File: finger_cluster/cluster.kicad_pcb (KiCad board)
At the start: 2 copper layers, 43.1 x 61 mm, 16 parts, among them J1 Conn_01x06_MountingPin, Q1 BSS84, SW1 SW_SPST, U1 TMAG5263

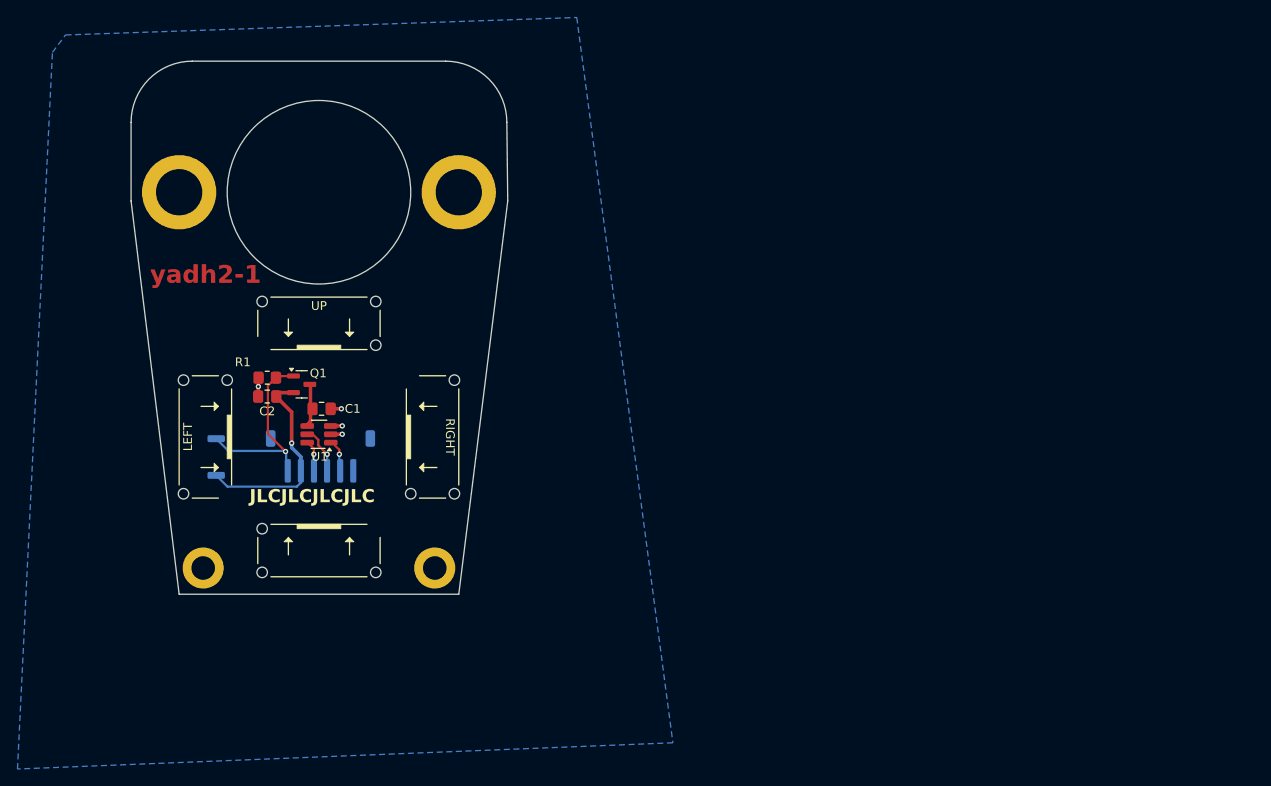
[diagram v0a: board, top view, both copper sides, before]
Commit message: cluster aluminium basic
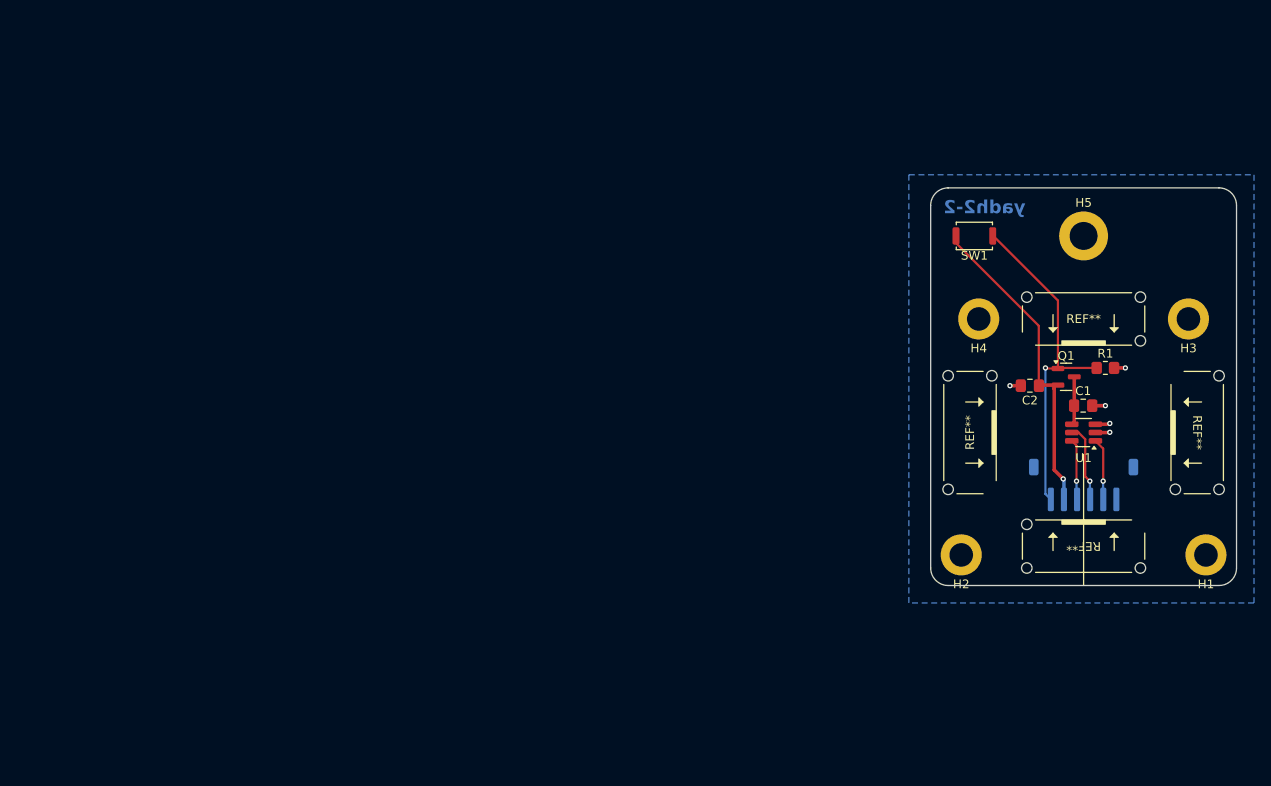
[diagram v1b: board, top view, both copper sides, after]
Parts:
- removed DOWN, LEFT, RIGHT, UP: key, cluster:key
- added H5: MountingHole_Pad, MountingHole:MountingHole_3.2mm_M3_DIN965_Pad, F.Cu at (187.5, 55.0)
- added REF**: key, cluster:key, F.Cu at (172.5, 77.5)
- added REF**: key, cluster:key, F.Cu at (187.5, 92.5)
- added REF**: key, cluster:key, F.Cu at (202.5, 77.5)
- added REF**: key, cluster:key, F.Cu at (187.5, 62.5)
- H1, H2: footprint MountingHole:MountingHole_5.3mm_M5_ISO14580_Pad -> MountingHole:MountingHole_2.7mm_M2.5_DIN965_Pad
- SW1: moved to F.Cu
- moved REF** 114.7 mm to (198.9, 55.4)
- moved H2 98.7 mm to (173.5, 91.5), turned to 180 degrees
- moved R1 95.9 mm to (190.0, 70.1), turned to 0 degrees
- moved H1 95.0 mm to (201.5, 91.5), turned to 180 degrees
- moved H4 93.2 mm to (175.5, 64.5), turned to 180 degrees
- moved H3 90.8 mm to (199.5, 64.5), turned to 180 degrees
- moved SW1 90.4 mm to (175.0, 55.0), turned to 180 degrees
- moved U1 87.5 mm to (187.5, 77.5)
- moved Q1 87.5 mm to (185.5, 71.1)
- moved J1 87.4 mm to (187.5, 83.5)
- moved C2 87.3 mm to (181.4, 72.1)
- moved C1 87.1 mm to (187.5, 74.4)
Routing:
- net /RST: track 22.6 -> 39.5 mm
- net +3.3V: track 23.6 -> 37.1 mm
- net /INT': track 5.67 -> 8.98 mm
- net /SDA: track 3.75 -> 6.95 mm
- net /SCL: track 3.93 -> 7.07 mm
- net GND: track 6.34 -> 7.39 mm, vias 4 -> 5
- net VDD: track 5.01 -> 5.95 mm
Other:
- board size 43.1 x 61 mm -> 35 x 45.5 mm
- board text added: "yadh2-2"
- board text removed: "JLCJLCJLCJLC"
- board text removed: "yadh2-1"
